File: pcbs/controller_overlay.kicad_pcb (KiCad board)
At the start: 2 copper layers, 19.7 x 60.1 mm, 2 parts

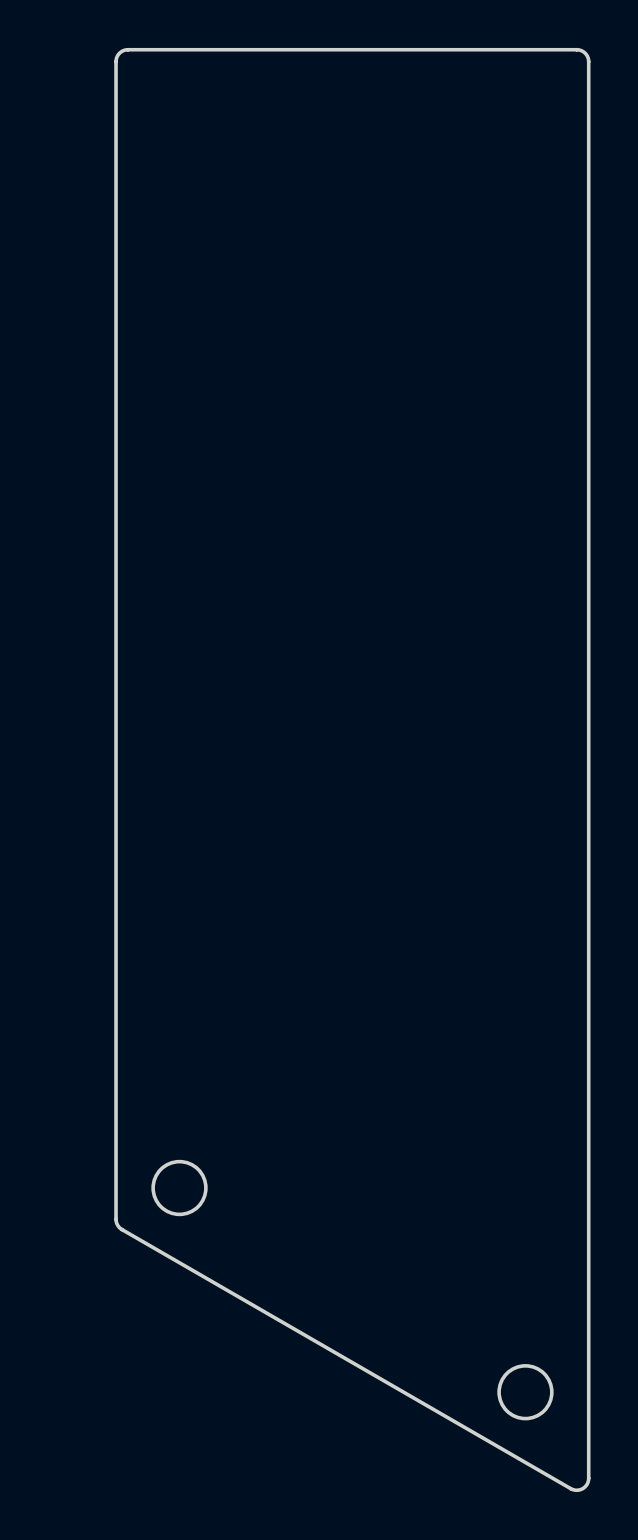
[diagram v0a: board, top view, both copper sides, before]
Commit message: feat: build script and its artifacts
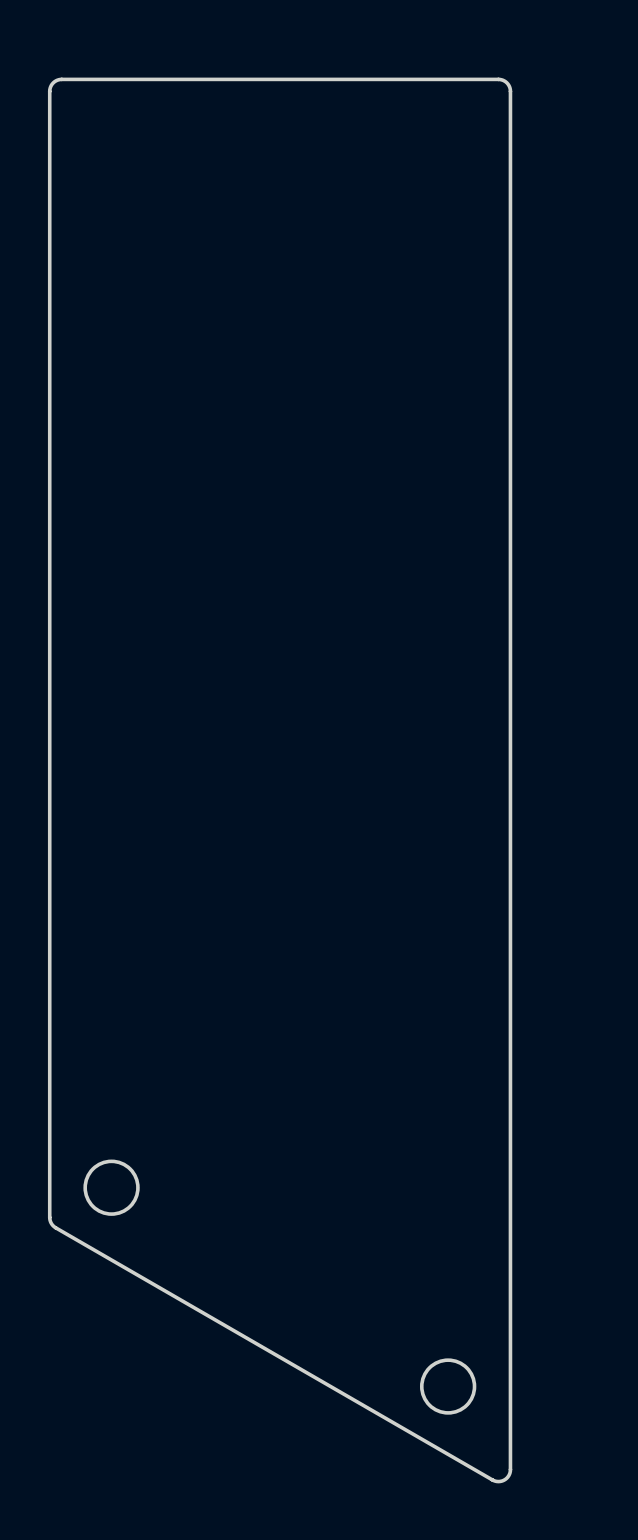
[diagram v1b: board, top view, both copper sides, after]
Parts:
- moved MH2 3.23 mm to (219.0, 108.8)
- moved MH1 2.84 mm to (204.9, 100.5)
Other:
- board size 19.7 x 60.1 mm -> 19.2 x 58.5 mm
